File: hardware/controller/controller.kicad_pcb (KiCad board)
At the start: 2 copper layers, 40.4 x 66.8 mm, 34 parts, among them J1 Screw_Terminal_01x02, J2 Screw_Terminal_01x02, J3 Screw_Terminal_01x02, J4 GROVE-CONNECTOR-DIP-90D_4P-2.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, J5 Screw_Terminal_01x03, T1 NMOSFETSOT23, T2 NMOSFETSOT23, T3 NMOSFETSOT23, T4 NMOSFETTO252, T5 NMOSFETTO252, U1 RO3.3-9S, U2 LM3480-5.0

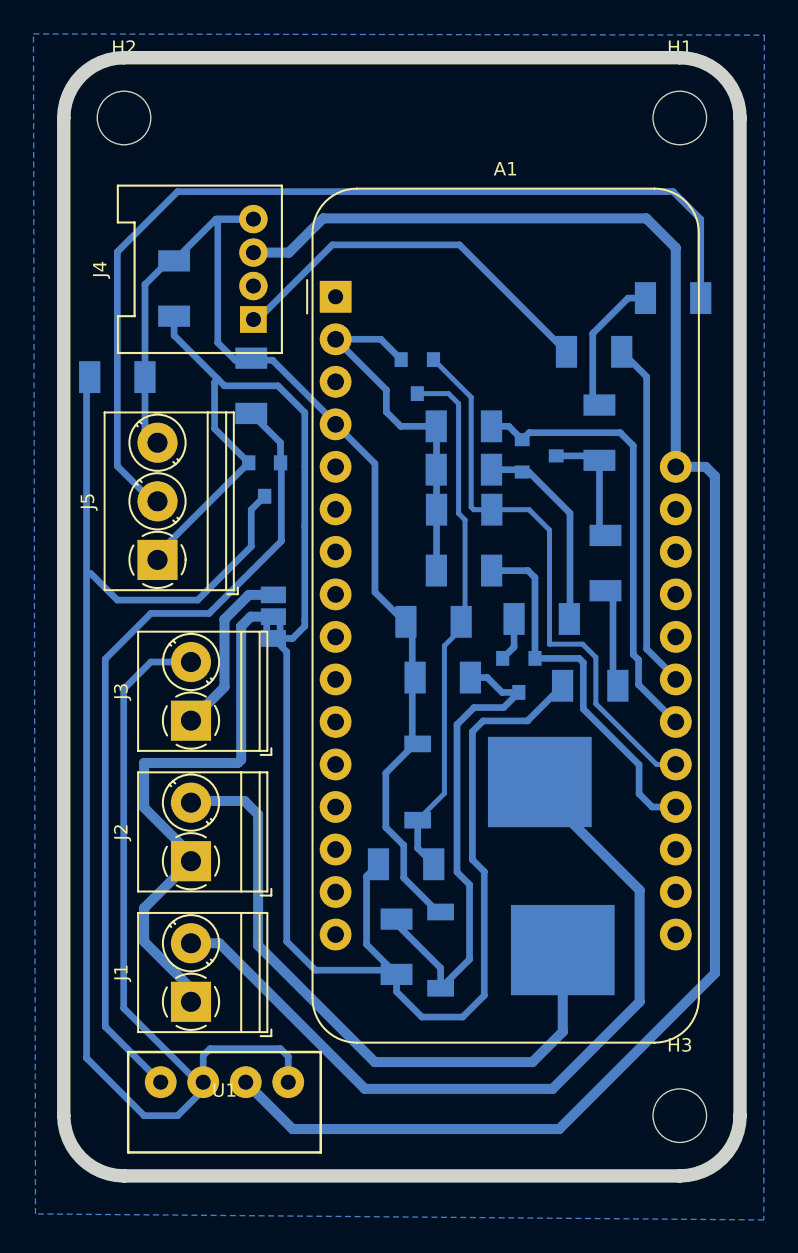
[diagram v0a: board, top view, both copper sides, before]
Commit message: Last version of controller
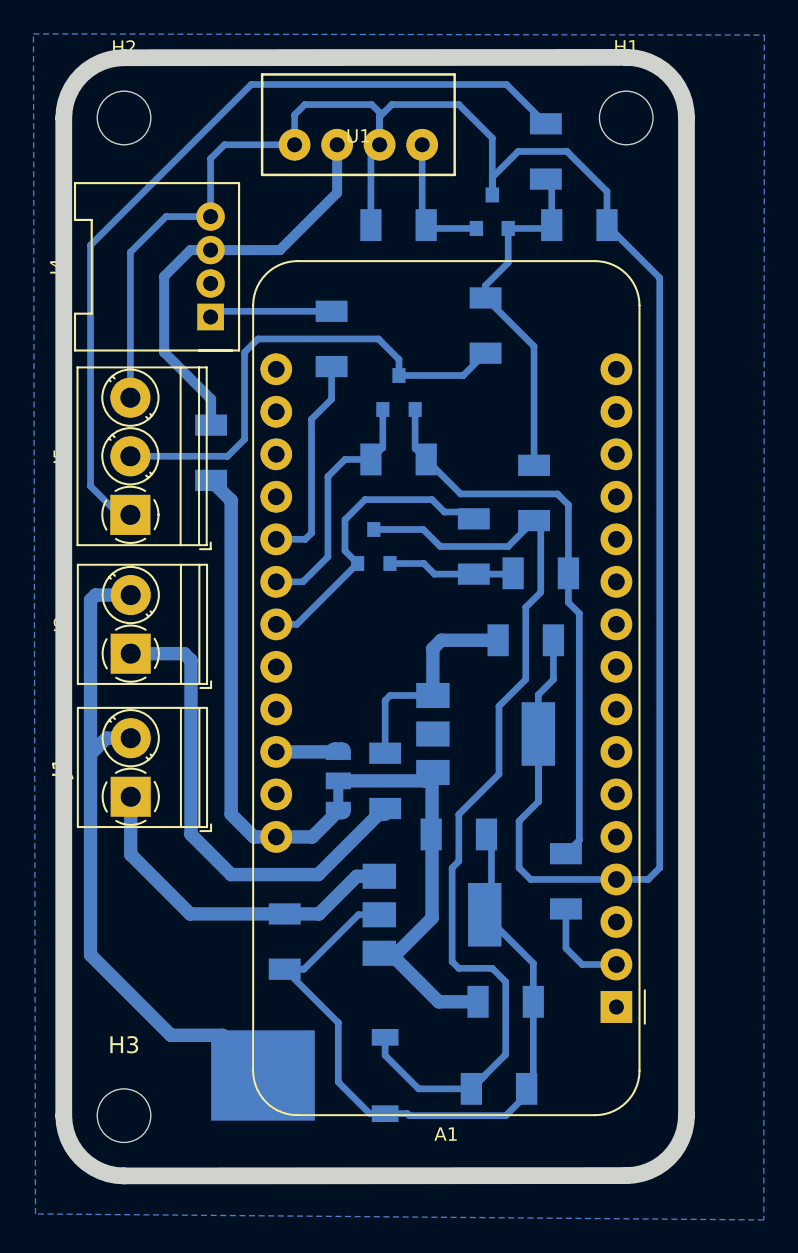
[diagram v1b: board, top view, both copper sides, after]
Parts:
- removed J3: Screw_Terminal_01x02, TerminalBlock_Phoenix:TerminalBlock_Phoenix_PT-1,5-2-3.5-H_1x02_P3.50mm_Horizontal
- removed R13, R15: 0, fab:fab-R1206FAB
- removed R4, R8: 10kΩ, fab:fab-R1206FAB
- removed T2: NMOSFETSOT23, fab:fab-SOT-23
- removed T5: NMOSFETTO252, fab:fab-TO252
- added C3: 1uF, fab:fab-C1206FAB, B.Cu at (140.8, 111.6)
- added C4: 4.7uF, fab:fab-C1206FAB, B.Cu at (142.0, 90.0)
- added C5: 1uF, fab:fab-C1206FAB, B.Cu at (138.0, 101.6)
- added C6: 4.7uF, fab:fab-C1206FAB, B.Cu at (127.6, 108.0)
- added U3: AP7361C-33E, Package_TO_SOT_SMD:SOT-223-3_TabPin2, B.Cu at (139.6, 95.6)
- added U4: AP7361C-33E, Package_TO_SOT_SMD:SOT-223-3_TabPin2, B.Cu at (136.4, 106.4)
- JP1: value SolderJumper_3_Bridged12 -> Jumper_3_Bridged12; footprint Jumper:SolderJumper-3_P1.3mm_Bridged2Bar12_Pad1.0x1.5mm -> Jumper:SolderJumper-3_P1.3mm_Bridged12_RoundedPad1.0x1.5mm
- R3: value 10kΩ -> 0
- moved U1 56.6 mm to (132.0, 60.4), turned to 180 degrees
- moved A1 45.6 mm to (147.4, 111.9), turned to 180 degrees
- moved H3 33.2 mm to (118.0, 118.4)
- moved R12 32.0 mm to (143.2, 60.8), turned to -90 degrees
- moved R2 28.3 mm to (142.5, 81.2), turned to -90 degrees
- moved R7 24.8 mm to (140.4, 116.8), turned to 0 degrees
- moved C2 24.5 mm to (145.2, 65.2), turned to 0 degrees
- moved R14 23.2 mm to (123.2, 78.8), turned to 90 degrees
- moved U2 21.0 mm to (140.0, 64.4), turned to 90 degrees
- moved R3 16.9 mm to (133.6, 98.4), turned to -90 degrees
- moved R6 15.9 mm to (139.6, 71.2), turned to -90 degrees
- moved R10 15.7 mm to (144.4, 104.4), turned to 90 degrees
- moved R9 15.7 mm to (130.4, 72.0), turned to -90 degrees
- moved T4 14.9 mm to (128.8, 116.0), turned to -90 degrees
- moved C1 13.0 mm to (134.4, 65.2), turned to 180 degrees
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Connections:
- net LIGHTMSFT_2_H renamed LIGHTMSFT_H
- A1 pad 20: LIGHTMSFT_2_L -> unconnected-(A1-Pad20)
- A1 pad 21: LIGHTMSFT_1_L -> Net-(A1-Pad21)
- A1 pad 23: Net-(A1-Pad23) -> LIGHTMSFT_L
- A1 pad 26: unconnected-(A1-Pad26) -> VBUS
- J1 pad 1: VOUT -> 3V3_REG_2
- J1 pad 2: LIGHTMSFT_1 -> LIGHTMSFT
- J2 pad 1: VOUT -> 3V3_REG_1
- J2 pad 2: LIGHTMSFT_2 -> LIGHTMSFT
- JP1 pad 1: 5V -> VBAT
- JP1 pad 2: VOUT -> VI
- JP1 pad 3: VIN -> VBUS
- R1 pad 2: LIGHTMSFT_2_L -> LIGHTMSFT_L
- R14 pad 1: LASERPWM_H -> VBAT
- R14 pad 2: LASERPWM_H -> VBAT
- R3 pad 1: 3V3 -> Net-(C4-Pad1)
- R3 pad 2: LIGHTMSFT_1_L -> 3V3_REG_1
- R9 pad 2: Net-(A1-Pad23) -> Net-(A1-Pad21)
- T1 pad 2: LIGHTMSFT_2_L -> LIGHTMSFT_L
- T4 pad 3: LIGHTMSFT_2 -> LIGHTMSFT
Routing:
- net VBAT: track 105.4 -> 53.4 mm
- net LIGHTMSFT_1: track 48.2 -> 0.00 mm
- net LASERPWM_H: track 73.6 -> 29.2 mm
- net Net-(C1-Pad1): track 48.5 -> 7.98 mm
- net LIGHTMSFT: track 0.00 -> 39.8 mm
- net LIGHTMSFT_2: track 38.9 -> 0.00 mm
- net 5V: track 109.2 -> 71.1 mm
- net LIGHTMSFT_1_L: track 34.0 -> 0.00 mm
- net VOUT: track 33.8 -> 0.00 mm
- net LIGHTMSFT_1_H: track 32.0 -> 0.00 mm
- net 3V3_REG_1: track 0.00 -> 28.3 mm
- net LIGHTMSFT_H: track 29.7 -> 58.0 mm
- net VI: track 0.00 -> 25.7 mm
- net LIGHTMSFT_2_L: track 22.3 -> 0.00 mm
- net Net-(A1-Pad23): track 20.9 -> 0.00 mm
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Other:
- board size 40.4 x 66.8 mm -> 37.2 x 66.8 mm
